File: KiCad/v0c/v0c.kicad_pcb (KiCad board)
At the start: 2 copper layers, 90 x 56.8 mm, 25 parts, among them U1 AM29F160, U10 IS62C256AL, U2 74HC139, U3 74HC273, U4 74HC191, U5 74HC191, U6 74HC191, U7 74HC670, U8 74HC00, U9 IS62C256AL

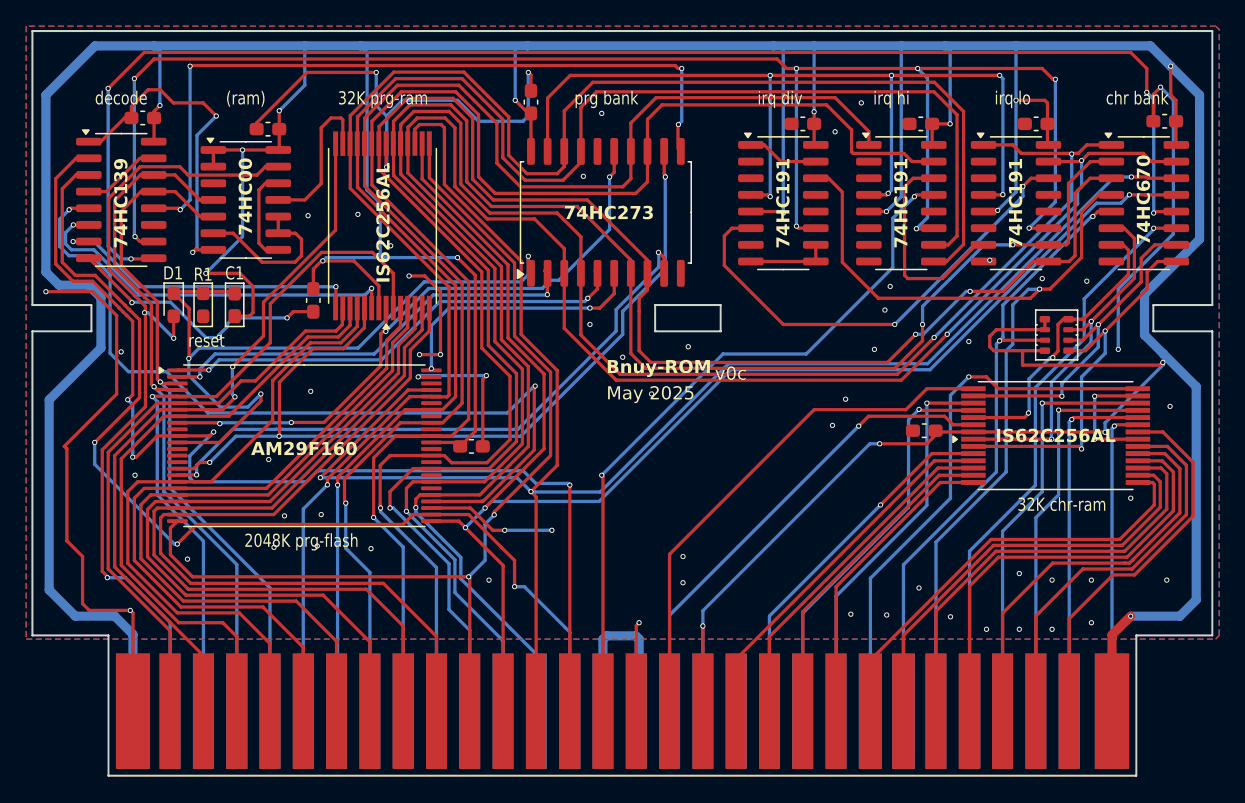
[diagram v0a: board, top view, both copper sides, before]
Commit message: sam2695 on board
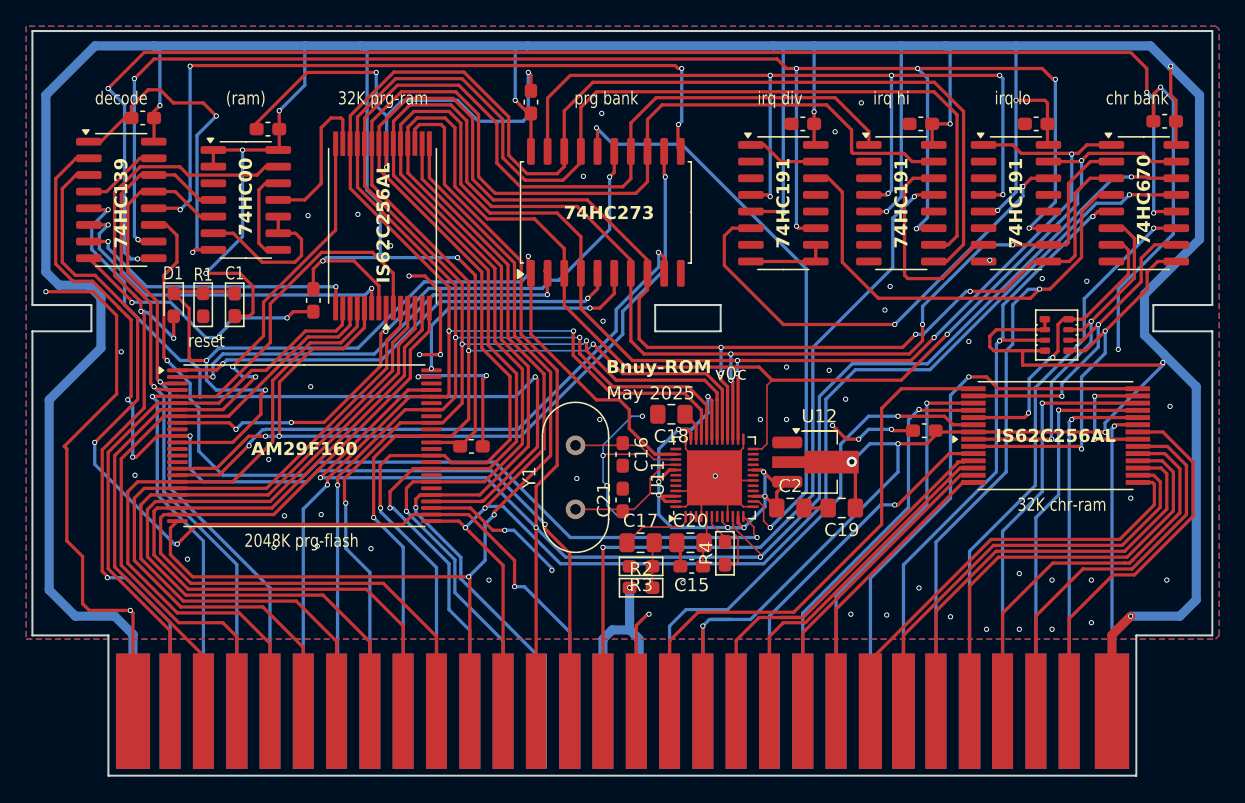
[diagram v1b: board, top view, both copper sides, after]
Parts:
- added C15: C_Small, Capacitor_SMD:C_0603_1608Metric_Pad1.08x0.95mm_HandSolder, F.Cu at (146.3, 113.0)
- added C16: C_Small, Capacitor_SMD:C_0603_1608Metric_Pad1.08x0.95mm_HandSolder, F.Cu at (141.0, 104.4)
- added C17: 1µF, Capacitor_SMD:C_0805_2012Metric_Pad1.18x1.45mm_HandSolder, F.Cu at (142.4, 111.2)
- added C18: C_Small, Capacitor_SMD:C_0805_2012Metric_Pad1.18x1.45mm_HandSolder, F.Cu at (144.7, 101.3)
- added C19: 1µF, Capacitor_SMD:C_0805_2012Metric_Pad1.18x1.45mm_HandSolder, F.Cu at (157.7, 108.5)
- added C2: 1µF, Capacitor_SMD:C_0805_2012Metric_Pad1.18x1.45mm_HandSolder, F.Cu at (153.8, 108.5)
- added C20: C_Small, Capacitor_SMD:C_0805_2012Metric_Pad1.18x1.45mm_HandSolder, F.Cu at (146.2, 111.2)
- added C21: C_Small, Capacitor_SMD:C_0603_1608Metric_Pad1.08x0.95mm_HandSolder, F.Cu at (141.0, 107.9)
- added R2: 100Ω, PCM_Resistor_SMD_AKL:R_0603_1608Metric_Pad1.05x0.95mm_HandSolder, F.Cu at (142.4, 114.6)
- added R3: 47KΩ, PCM_Resistor_SMD_AKL:R_0603_1608Metric_Pad1.05x0.95mm_HandSolder, F.Cu at (142.4, 113.0)
- added R4: 4.7K, PCM_Resistor_SMD_AKL:R_0603_1608Metric_Pad1.05x0.95mm_HandSolder, F.Cu at (148.8, 112.0)
- added U11: SAM2695, Package_DFN_QFN:QFN-48-1EP_6x6mm_P0.4mm_EP4.2x4.2mm, F.Cu at (148.0, 106.2)
- added U12: MCP1700, Package_TO_SOT_SMD:SOT-89-3_Handsoldering, F.Cu at (156.0, 105.0)
- added Y1: 12M, Crystal:Crystal_HC49-4H_Vertical, F.Cu at (137.4, 108.6)
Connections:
- net Net-(H1-cAUDIO) renamed /rfAUDIO
- U3 pad 16: /~{SAMCS} -> /~{SoundCS}
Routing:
- net /~{samWr}: track 0.00 -> 68.3 mm, vias 0 -> 2
- net GND: track 210.5 -> 266.7 mm, vias 69 -> 76
- net +3V3: track 0.00 -> 46.1 mm, vias 0 -> 8
- net /~{SoundCS}: track 0.00 -> 46.0 mm, vias 0 -> 2
- net /cD7: track 127.2 -> 152.5 mm, vias 1 -> 3
- net /cD5: track 106.6 -> 131.9 mm, vias 1 -> 3
- net /cD4: track 112.6 -> 137.4 mm, vias 1 -> 3
- net /cD6: track 123.0 -> 147.6 mm, vias 1 -> 3
- net /~{RESET}: track 58.4 -> 78.0 mm
- net /cA0: track 139.0 -> 151.5 mm, vias 3 -> 4
- net VCC: track 459.6 -> 469.4 mm, vias 19 -> 20
- net Net-(U11-X2): track 0.00 -> 9.72 mm
- net /cA1: track 115.9 -> 124.1 mm
- net Net-(U11-X1): track 0.00 -> 8.10 mm
- net /R~{W}: track 86.4 -> 80.1 mm
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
